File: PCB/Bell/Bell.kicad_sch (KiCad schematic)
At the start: 38 parts, among them J1 USB-C, J2 POWER, J3 Conn_01x08, J4 Shelly, J5 Conn_01x05, J6 Conn_01x02, U1 ESP32-PICO-MINI-02, U2 FT231XQ, U3 ISL89410, U4 ISL89410, U5 LMR16006XDDCR, U7 AA, U8 QR

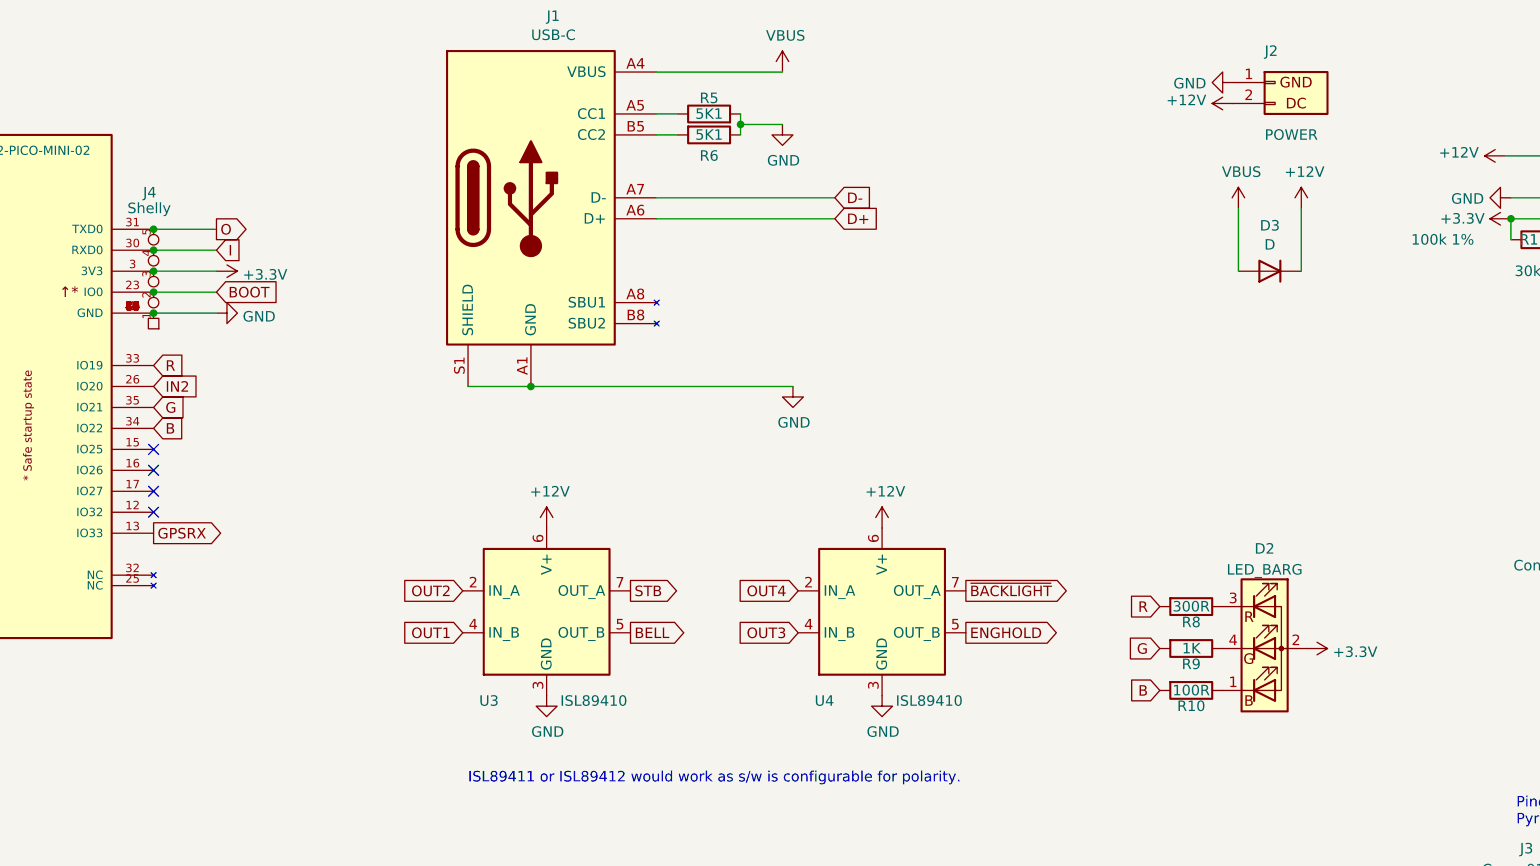
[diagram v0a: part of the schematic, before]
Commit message: Library update
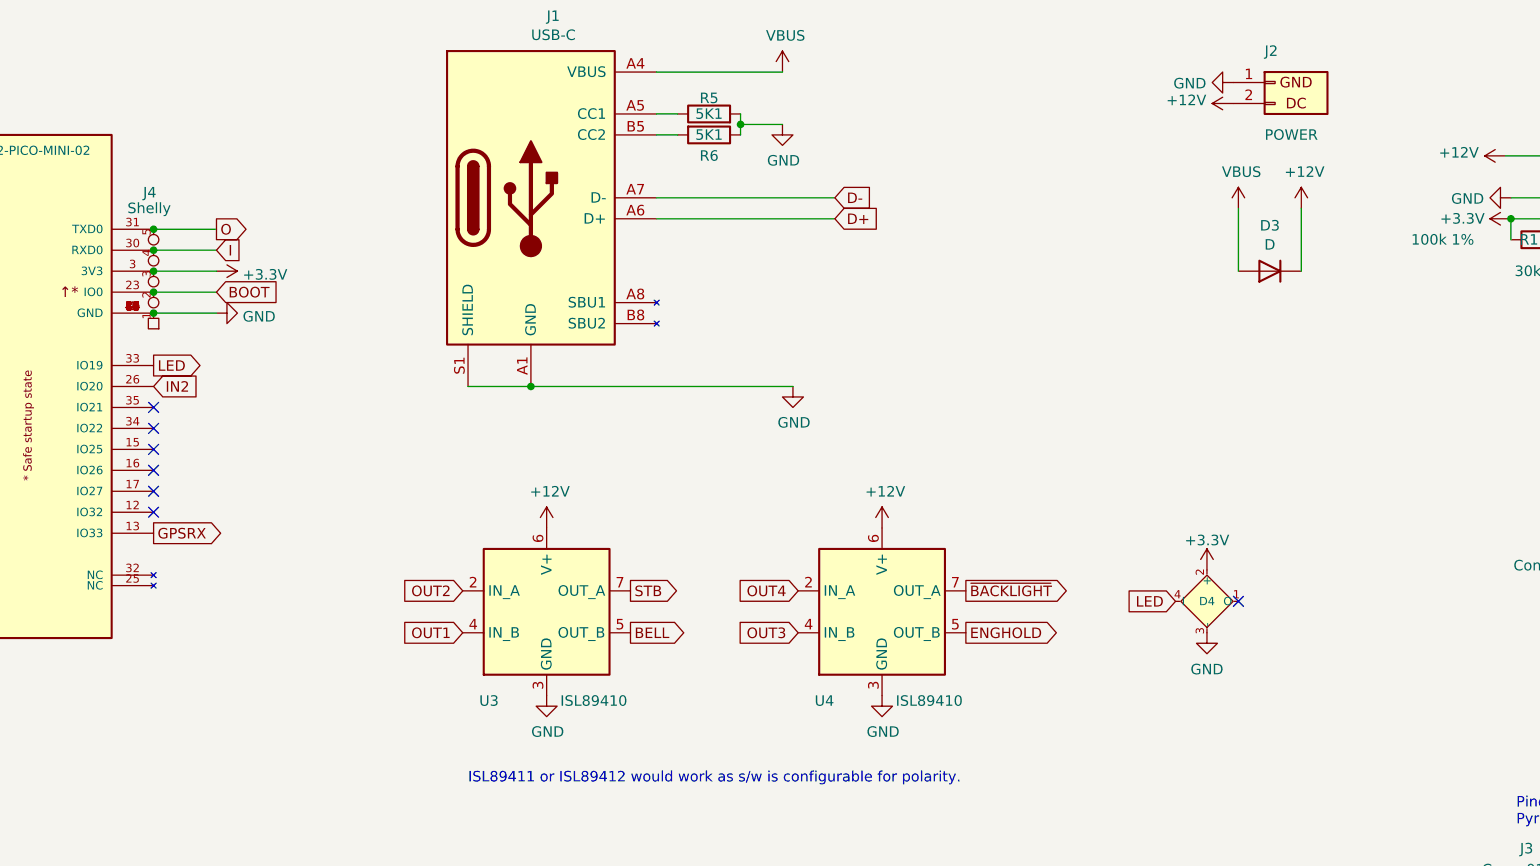
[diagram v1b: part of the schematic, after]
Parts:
- removed D2: LED_BARG, RevK:MHS190RGBCT, symbol Device:LED_BARG
- removed R10: 100R, RevK:R_0603, symbol Device:R
- removed R8: 300R, RevK:R_0603, symbol Device:R
- removed R9: 1K, RevK:R_0603, symbol Device:R
- added D4: XL-1010RGBC-WS2812B, RevK:SMD1010, symbol RevK:WS2812B-1mm
- U1: LCSC Part # (none) -> C2980306
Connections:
- net +3V3: now also D4.2 (+)
- net GND: now also D4.3 (-)
- net B: no longer names the net of U1.34 (IO22)
- net G: no longer names the net of U1.35 (IO21)
- net R renamed LED
- net LED: now also D4.4 (I)
- no-connect marks 15 -> 18

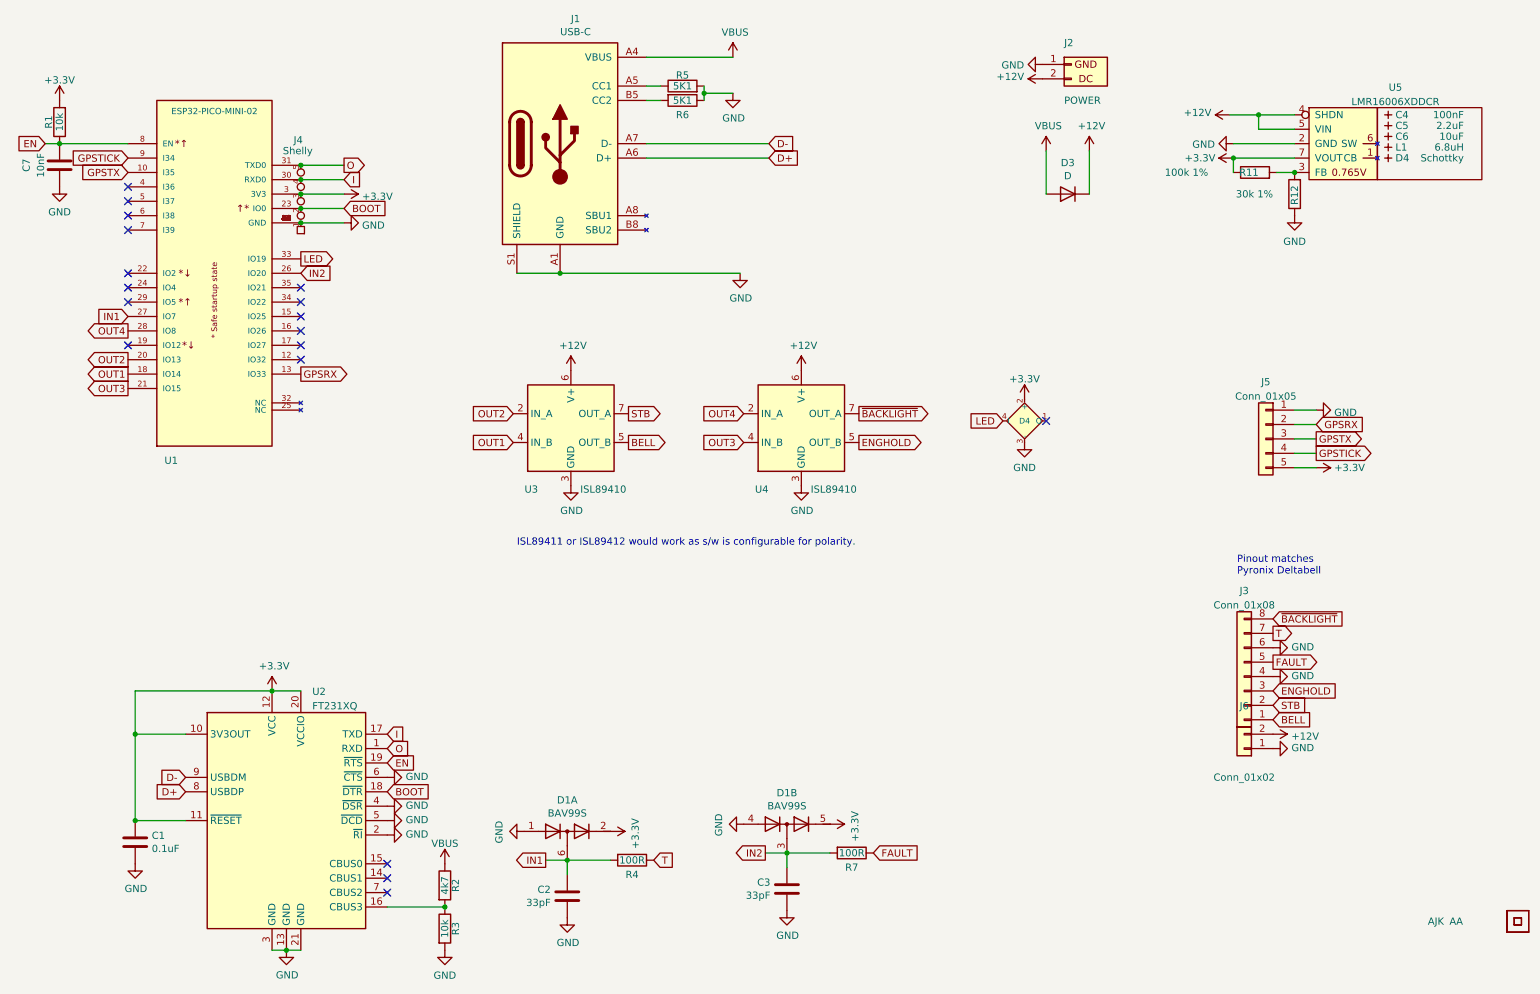
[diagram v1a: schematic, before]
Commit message: S3
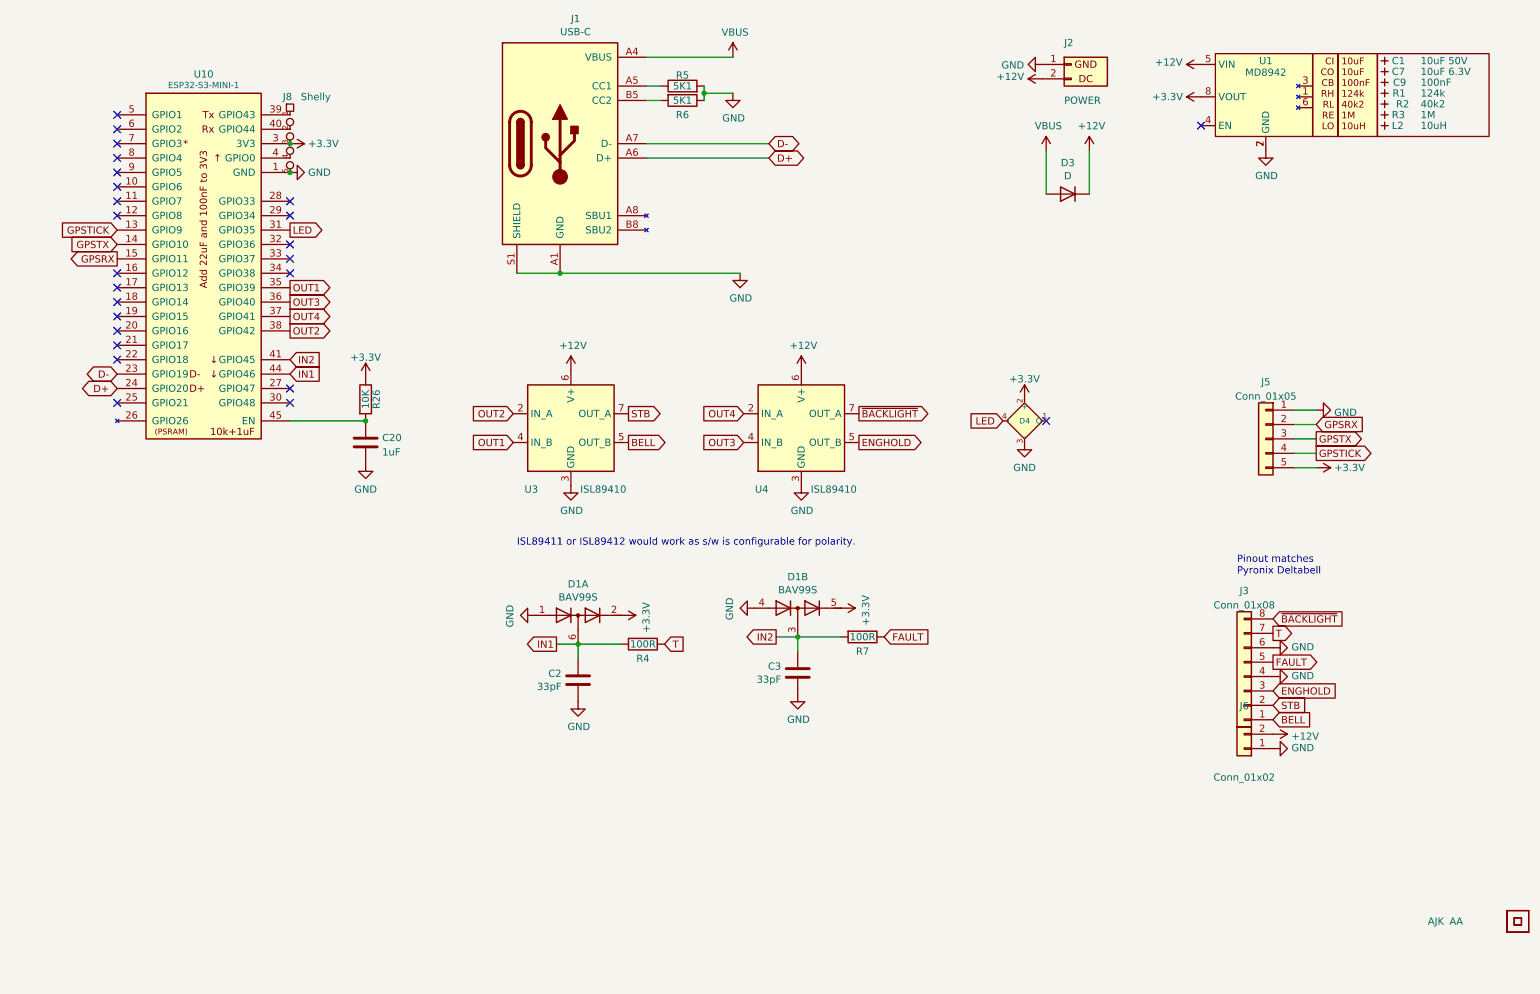
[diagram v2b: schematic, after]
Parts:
- removed C1: 0.1uF, RevK:C_0603, symbol Device:C
- removed C4: 100nF, RevK:C_0603_, symbol RevK:Hidden
- removed C5: 2.2uF, RevK:C_0805_, symbol RevK:Hidden
- removed C6: 10uF, RevK:C_0805_, symbol RevK:Hidden
- removed C7: 10nF, RevK:C_0603, symbol Device:C
- removed D4: Schottky, RevK:D_1206_, symbol RevK:Hidden
- removed J4: Shelly, RevK:Shelly, symbol RevK:Shelly
- removed L1: 6.8uH, RevK:L_4x4_, symbol RevK:Hidden
- removed R1, R3: 10k, RevK:R_0603, symbol Device:R
- removed R11: 100k 1%, RevK:R_0603, symbol Device:R
- removed R12: 30k 1%, RevK:R_0603, symbol Device:R
- removed R2: 4k7, RevK:R_0603, symbol Device:R
- removed U1: ESP32-PICO-MINI-02, RevK:ESP32-PICO-MINI-02, symbol RevK:ESP32-PICO-MINI-02
- removed U2: FT231XQ, RevK:QFN-20-1EP_4x4mm_P0.5mm_EP2.5x2.5mm, symbol RevK:FT231XQ
- removed U5: LMR16006XDDCR, RevK:SOT-23-Thin-6-Reg, symbol RevK:LMR16006XDDCR
- added C1: 10uF 50V, RevK:C_0603_, symbol RevK:Hidden
- added C20: 1uF, RevK:C_0402, symbol Device:C
- added C7: 10uF 6.3V, RevK:C_0603_, symbol RevK:Hidden
- added C9: 100nF, RevK:C_0603_, symbol RevK:Hidden
- added J8: Shelly, RevK:Shelly, symbol RevK:Shelly
- added L2: 10uH, RevK:L_4x4_, symbol RevK:Hidden
- added R1: 124k, RevK:R_0402_, symbol RevK:Hidden
- added R2: 40k2, RevK:R_0402_, symbol RevK:Hidden
- added R26: 10K, RevK:R_0402, symbol Device:R
- added R3: 1M, RevK:R_0402_, symbol RevK:Hidden
- added U1: MD8942, RevK:SOT-23-6-MD8942, symbol RevK:MD89420-RegBlock
- added U10: ESP32-S3-MINI-1, RevK:ESP32-S3-MINI-1, symbol RevK:ESP32-S3-MINI-1-N4R2
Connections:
- net +12V: now also U1.5 (VIN)
- net +3V3: now also J8.3 (3V3), R26.1, U1.8 (VOUT), U10.3 (3V3)
- net D+: now also U10.24 (GPIO20)
- net D-: now also U10.23 (GPIO19)
- net GND: now also C20.2, J8.5 (Tx), U1.2 (GND), U1.7 (GND), U10.1 (GND), U10.2 (GND), U10.42 (GND), U10.43 (GND), U10.46 (GND), U10.47 (GND), U10.48 (GND), U10.49 (GND), U10.50 (GND), U10.51 (GND), U10.52 (GND), U10.53 (GND), U10.54 (GND), U10.55 (GND), U10.56 (GND), U10.57 (GND), U10.58 (GND), U10.59 (GND), U10.60 (GND), U10.61 (GND), U10.62 (GND), U10.63 (GND), U10.64 (GND), U10.65 (GND)
- net GPSRX: now also U10.15 (GPIO11)
- net GPSTICK: now also U10.13 (GPIO9)
- net GPSTX: now also U10.14 (GPIO10)
- net IN1: now also U10.44 (GPIO46)
- net IN2: now also U10.41 (GPIO45)
- net LED: now also U10.31 (GPIO35)
- net OUT1: now also U10.35 (GPIO39)
- net OUT2: now also U10.38 (GPIO42)
- net OUT3: now also U10.36 (GPIO40)
- net OUT4: now also U10.37 (GPIO41)
- new net: C20.1, R26.2, U10.45 (EN)
- new net: J8.1 (GND), U10.39 (GPIO43)
- new net: J8.4 (Rx), U10.4 (GPIO0)
- new net: J8.2 (0), U10.40 (GPIO44)
- no-connect marks 18 -> 25
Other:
- moved on the sheet: C2, C3, D1A, D1B, R4, R7

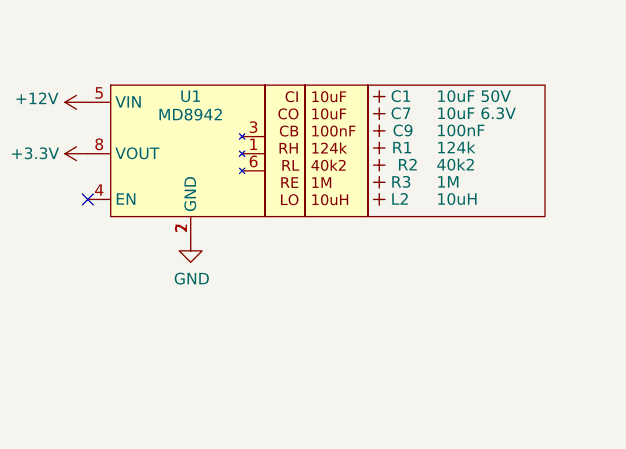
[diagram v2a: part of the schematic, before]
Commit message: Clean up a lot
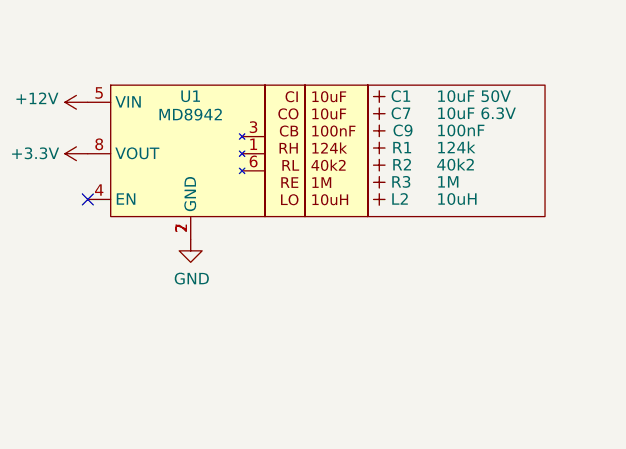
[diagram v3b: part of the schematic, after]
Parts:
- C2, C3: footprint RevK:C_0603 -> RevK:C_0402
- D1: footprint Package_TO_SOT_SMD:SOT-363_SC-70-6 -> RevK:SOT-363_SC-70-6
- R4, R5, R6, R7: footprint RevK:R_0603 -> RevK:R_0402
- U3, U4: footprint Package_SO:SO-8_3.9x4.9mm_P1.27mm -> RevK:SO-8_3.9x4.9mm_P1.27mm
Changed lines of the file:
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@@
       (effects (font (size 1.27 1.27)))
     )
-    (property "Footprint" "RevK:R_0603" (at 133.35 29.718 90)
+    (property "Footprint" "RevK:R_0402" (at 133.35 29.718 90)
       (effects (font (size 1.27 1.27)) hide)
     )
@@
       (effects (font (size 1.27 1.27)))
     )
-    (property "Footprint" "RevK:R_0603" (at 133.35 28.702 90)
+    (property "Footprint" "RevK:R_0402" (at 133.35 28.702 90)
       (effects (font (size 1.27 1.27)) hide)
     )
@@
       (effects (font (size 1.27 1.27)))
     )
-    (property "Footprint" "RevK:R_0603" (at 126.365 124.587 90)
+    (property "Footprint" "RevK:R_0402" (at 126.365 124.587 90)
       (effects (font (size 1.27 1.27)) hide)
     )
@@
       (effects (font (size 1.27 1.27)) (justify left))
     )
-    (property "Footprint" "RevK:C_0603" (at 113.9698 136.525 0)
+    (property "Footprint" "RevK:C_0402" (at 113.9698 136.525 0)
       (effects (font (size 1.27 1.27)) hide)
     )
@@
       (effects (font (size 1.27 1.27)))
     )
-    (property "Footprint" "Package_TO_SOT_SMD:SOT-363_SC-70-6" (at 114.935 133.985 0)
+    (property "Footprint" "RevK:SOT-363_SC-70-6" (at 114.935 133.985 0)
       (effects (font (size 1.27 1.27)) hide)
     )
     (property "Datasheet" "https://assets.nexperia.com/documents/data-sheet/BAV99_SER.pdf" (at 114.935 121.285 0)
+      (effects (font (size 1.27 1.27)) hide)
+    )
+    (property "Field4" "" (at 114.935 121.285 0)
       (effects (font (size 1.27 1.27)) hide)
     )
@@
       (effects (font (size 1.27 1.27)))
     )
-    (property "Footprint" "RevK:R_0603" (at 165.1 123.317 90)
+    (property "Footprint" "RevK:R_0402" (at 165.1 123.317 90)
       (effects (font (size 1.27 1.27)) hide)
     )
@@
       (effects (font (size 1.27 1.27)) (justify left))
     )
-    (property "Footprint" "RevK:C_0603" (at 152.7048 135.255 0)
+    (property "Footprint" "RevK:C_0402" (at 152.7048 135.255 0)
       (effects (font (size 1.27 1.27)) hide)
     )
@@
       (effects (font (size 1.27 1.27)))
     )
-    (property "Footprint" "Package_TO_SOT_SMD:SOT-363_SC-70-6" (at 153.67 132.715 0)
+    (property "Footprint" "RevK:SOT-363_SC-70-6" (at 153.67 132.715 0)
       (effects (font (size 1.27 1.27)) hide)
     )
     (property "Datasheet" "https://assets.nexperia.com/documents/data-sheet/BAV99_SER.pdf" (at 153.67 120.015 0)
+      (effects (font (size 1.27 1.27)) hide)
+    )
+    (property "Field4" "" (at 153.67 120.015 0)
       (effects (font (size 1.27 1.27)) hide)
     )
@@
       (effects (font (size 1.27 1.27)))
     )
-    (property "Footprint" "Package_SO:SO-8_3.9x4.9mm_P1.27mm" (at 113.665 95.885 0)
+    (property "Footprint" "RevK:SO-8_3.9x4.9mm_P1.27mm" (at 113.665 95.885 0)
       (effects (font (size 1.27 1.27)) hide)
     )
@@
       (effects (font (size 1.27 1.27)))
     )
-    (property "Footprint" "Package_SO:SO-8_3.9x4.9mm_P1.27mm" (at 154.305 95.885 0)
+    (property "Footprint" "RevK:SO-8_3.9x4.9mm_P1.27mm" (at 154.305 95.885 0)
       (effects (font (size 1.27 1.27)) hide)
     )
@@
   (symbol (lib_id "RevK:Hidden") (at 257.175 31.115 270) (unit 1)
     (in_bom yes) (on_board yes) (dnp no)
-    (property "Reference" "R2" (at 260.35 31.115 90)
-      (effects (font (size 1.27 1.27)))
-    )
+    (property "Reference" "R2" (at 259.715 31.115 90)
+      (effects (font (size 1.27 1.27)))
+    )
